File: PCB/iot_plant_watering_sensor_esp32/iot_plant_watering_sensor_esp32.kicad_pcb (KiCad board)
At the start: 2 copper layers, 140.8 x 18.1 mm, 19 parts, among them Q1 2N7002P,215, SW1 SW_Push_KMR2, U1 ESP32-WROOM-32, U2 HT7830

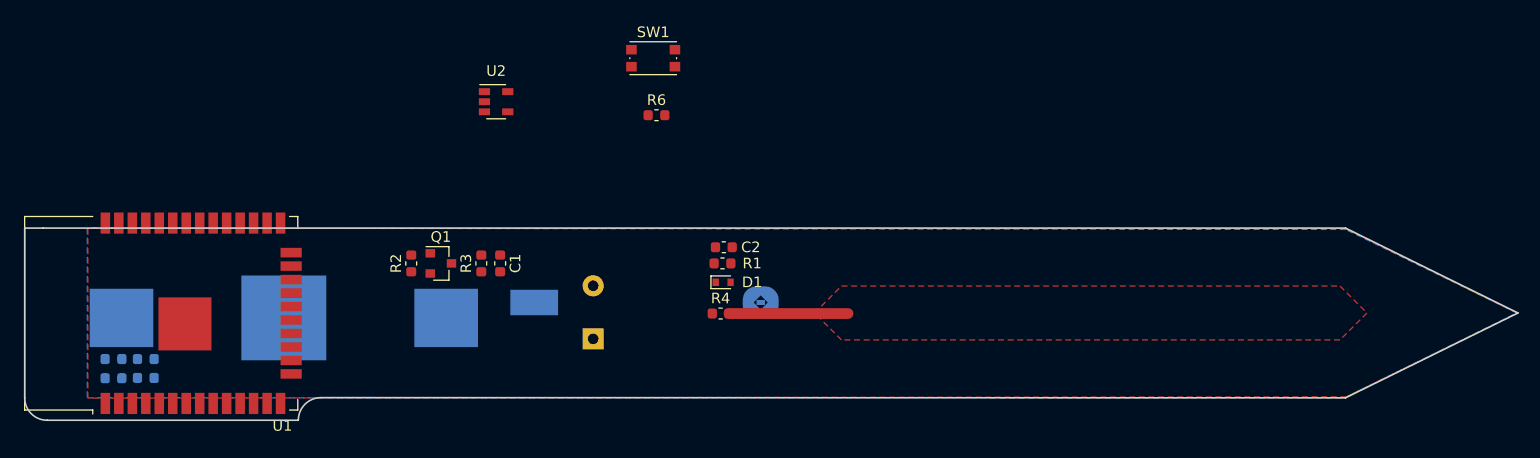
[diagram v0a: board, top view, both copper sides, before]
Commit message: pcb release
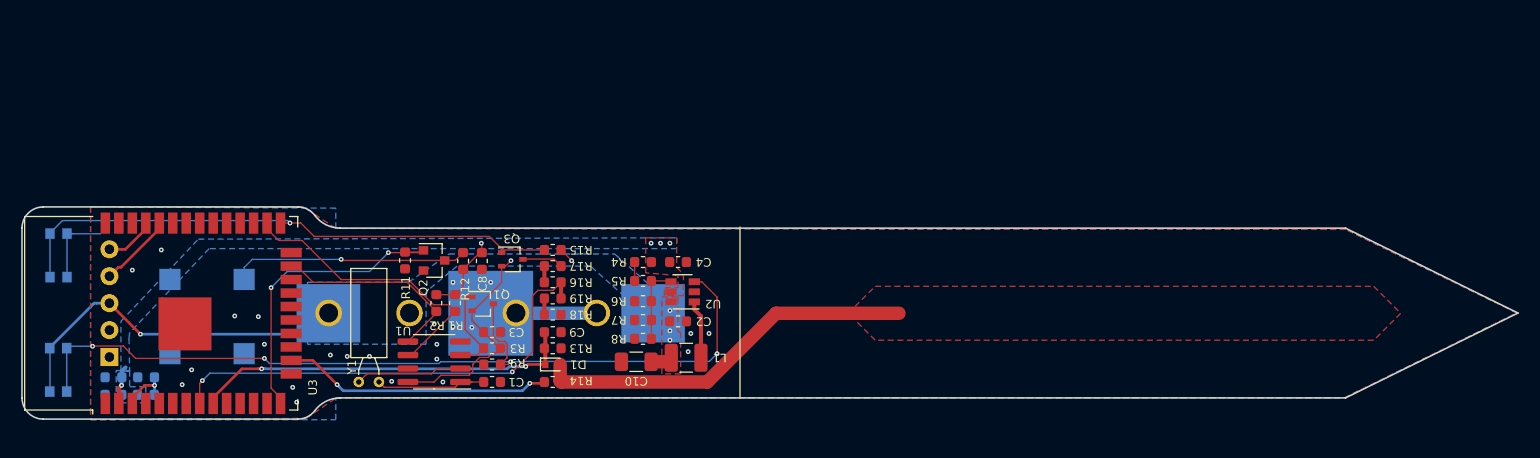
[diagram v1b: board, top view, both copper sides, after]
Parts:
- added C1: 25p, Capacitor_SMD:C_0603_1608Metric, F.Cu at (122.6, 111.5)
- added C10: 100u, Capacitor_SMD:C_1206_3216Metric, F.Cu at (136.1, 109.6)
- added C4: 10u, Capacitor_SMD:C_0603_1608Metric, F.Cu at (140.1, 100.2)
- added C7: 10u, Capacitor_SMD:C_0603_1608Metric, B.Cu at (86.9, 111.1)
- added C9: 1u, Capacitor_SMD:C_0603_1608Metric, F.Cu at (128.3, 106.8)
- added CONFIG1: SW_Push_KMR2, SamacSys_Parts:SW_Push_1P1T_NO_CK_KMR2, B.Cu at (81.7, 110.4)
- added J1: Conn_01x05, custom:PinHeader_1x05_P2.54mm_Snuggly, B.Cu at (86.5, 109.2)
- added L1: 4.7u, Inductor_SMD:L_1210_3225Metric, F.Cu at (140.8, 109.2)
- added Q1: BSS84W-7-F, Package_TO_SOT_SMD:SOT-323_SC-70, F.Cu at (121.7, 104.1)
- added Q3: BSS84W-7-F, Package_TO_SOT_SMD:SOT-323_SC-70, F.Cu at (124.5, 99.9)
- added R11: 10K, Resistor_SMD:R_0603_1608Metric, F.Cu at (114.4, 100.1)
- added R13: 510K, Resistor_SMD:R_0603_1608Metric, F.Cu at (128.3, 108.3)
- added R14: 10K, Resistor_SMD:R_0603_1608Metric, F.Cu at (128.3, 111.5)
- added R15: 10K, Resistor_SMD:R_0603_1608Metric, F.Cu at (128.3, 99.1)
- added R16: 510K, Resistor_SMD:R_0603_1608Metric, F.Cu at (128.3, 100.6)
- added R17: 510K, Resistor_SMD:R_0603_1608Metric, F.Cu at (128.3, 102.1)
- added R18: 510K, Resistor_SMD:R_0603_1608Metric, F.Cu at (128.3, 103.6)
- added R19: 510K, Resistor_SMD:R_0603_1608Metric, F.Cu at (128.3, 105.2)
- added R3: 10K, Resistor_SMD:R_0603_1608Metric, F.Cu at (122.6, 108.3)
- added R5: 510K, Resistor_SMD:R_0603_1608Metric, F.Cu at (136.8, 102.0)
- added R7: 510K, Resistor_SMD:R_0603_1608Metric, F.Cu at (136.8, 105.7)
- added R8: 510K, Resistor_SMD:R_0603_1608Metric, F.Cu at (136.8, 107.4)
- added R9: 10K, Resistor_SMD:R_0603_1608Metric, F.Cu at (122.6, 109.9)
- added U1: PCF8563T, Package_SO:SOIC-8_3.9x4.9mm_P1.27mm, F.Cu at (117.1, 109.6)
- added Y1: 32.768 kHz, Crystal:Crystal_C38-LF_D3.0mm_L8.0mm_Horizontal, F.Cu at (111.9, 111.5)
- BOOT1: renamed from SW1; moved to B.Cu
- BT2: value CR2032 -> CR2; footprint custom:BS-8-1 -> custom:2915_CR2
- BUZZER1: renamed from LS1; value PS1240P02BT -> FUET-8530H-3.6V; footprint Buzzer_Beeper:Buzzer_TDK_PS1240P02BT_D12.2mm_H6.5mm -> Buzzer_Beeper:PUIAudio_SMT_0825_S_4_R
- C2: value 1u -> 10u
- C3: moved to F.Cu
- C5: value 10u -> 100n
- R1: value 510K -> 10K
- R4, R6: value 10K -> 510K
- U2: value HT7830 -> FP6714; footprint Package_TO_SOT_SMD:SOT-23-5 -> Package_TO_SOT_SMD:SOT-23-6
- moved BOOT1 59.1 mm to (81.7, 99.6), turned to 90 degrees
- moved BUZZER1 36.5 mm to (95.7, 105.3), turned to 270 degrees
- moved C3 32.9 mm to (122.6, 106.8), turned to 0 degrees
- moved R1 25.5 mm to (119.1, 104.1), turned to 90 degrees
- moved U2 25.1 mm to (140.5, 103.0), turned to 180 degrees
- moved BT1 19.5 mm to (122.4, 105.0)
- moved D1 17.8 mm to (128.3, 109.9)
- moved R6 17.6 mm to (136.8, 103.9), turned to 180 degrees
- moved BT2 15.1 mm to (119.8, 105.0)
- moved R4 8.78 mm to (136.8, 100.2), turned to 180 degrees
- moved C2 8.21 mm to (140.1, 105.8)
- moved R2 4.42 mm to (117.3, 104.1)
- moved C6 3.37 mm to (86.9, 112.7)
- moved R10 3.37 mm to (89.9, 112.7)
- moved C5 3.07 mm to (89.9, 111.1)
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- renumbered C4 to C6, C1 to C8, Q1 to Q2, R5 to R10, R3 to R12, U1 to U3
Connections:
- BOOT1 pad 1: Net-(SW1-Pad1) -> GND
- BOOT1 pad 2: Net-(SW1-Pad2) -> BOOT
- BT1 pad 1: Net-(BT1-Pad1) -> +BATT
- BT2 pad 1: (no net) -> +BATT
- BT2 pad 2: (no net) -> GND
- BUZZER1 pad 1: +3V0 -> +3V3
- C2 pad 1: C_SENSE -> +BATT
- C3 pad 1: Net-(C3-Pad1) -> +BATT
- C5 pad 1: +3V0 -> Net-(C5-Pad1)
- C6 pad 1: +3V0 -> +3V3
- C8 pad 1: (no net) -> +3V3
- R1 pad 1: C_SENSE -> SCL
- R1 pad 2: GND -> +3V3
- R10 pad 1: Net-(C3-Pad1) -> Net-(C5-Pad1)
- R10 pad 2: +3V0 -> +3V3
- R12 pad 1: +3V0 -> +3V3
- R2 pad 1: GND -> SDA
- R2 pad 2: BUZZER -> +3V3
- R4 pad 1: PWM -> +3V3
- R4 pad 2: /C_SENSOR+ -> Net-(R4-Pad2)
- R6 pad 1: (no net) -> FB
- R6 pad 2: (no net) -> GND
- U2 pad 1: (no net) -> Net-(L1-Pad2)
- U2 pad 3: (no net) -> LDO_EN
- U2 pad 4: (no net) -> FB
- U2 pad 5: (no net) -> +3V3
- U3 pad 10: BUZZER -> (no net)
- U3 pad 12: PWM -> (no net)
- U3 pad 14: (no net) -> BUZZER
- U3 pad 16: (no net) -> PWM
- U3 pad 2: +3V0 -> +3V3
- U3 pad 23: (no net) -> SDA
- U3 pad 25: (no net) -> BOOT
- U3 pad 26: (no net) -> SCL
- U3 pad 3: Net-(C3-Pad1) -> Net-(C5-Pad1)
- U3 pad 34: (no net) -> RXD
- U3 pad 35: (no net) -> TXD
- U3 pad 8: C_SENSE -> BATT_ADC
- U3 pad 9: (no net) -> C_SENSE
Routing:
- net LDO_EN: track 0.00 -> 82.6 mm, vias 0 -> 4
- net +BATT: track 0.00 -> 64.6 mm, vias 0 -> 6
- net BOOT: track 0.00 -> 53.8 mm, vias 0 -> 1
- net BATT_ADC: track 0.00 -> 44.5 mm, vias 0 -> 2
- net C_SENSE: track 0.00 -> 36.2 mm, vias 0 -> 2
- net BUZZER: track 0.00 -> 28.9 mm, vias 0 -> 2
- net SCL: track 0.00 -> 27.6 mm
- net PWM: track 0.00 -> 25.4 mm, vias 0 -> 2
- net /C_SENSOR+: track 11.2 -> 36.2 mm
- net Net-(BUZZER1-Pad2): track 0.00 -> 22.4 mm, vias 0 -> 1
- net SDA: track 0.00 -> 19.4 mm
- net GND: track 0.00 -> 17.3 mm, vias 0 -> 24
- net +3V3: track 0.00 -> 11.5 mm, vias 0 -> 5
- net Net-(C1-Pad1): track 0.00 -> 10.3 mm
- net Net-(U1-Pad2): track 0.00 -> 10.1 mm
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- added copper zone on B.Cu, net +3V3
- added copper zone on F.Cu, net +3V3
- added copper zone on B.Cu, net +BATT
- added copper zone on F.Cu, net +BATT
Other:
- board size 140.8 x 18.1 mm -> 141 x 20 mm
- net class C_SENSE added: clearance 0.127, trace_width 1.016, via_dia 0.45, via_drill 0.2
- net class Default: clearance 0.2 -> 0.127; trace_width 0.25 -> 0.127; via_dia 0.8 -> 0.45; via_drill 0.4 -> 0.2
- rule trace_clearance: 0.2 -> 0.127
- rule trace_min: 0.2 -> 0
- rule via_min_drill: 0.3 -> 0.2
- rule via_min_size: 0.4 -> 0.45
- board text added: "Leonardo Bispo github.com/ldab rev1 - Nov-2020"
